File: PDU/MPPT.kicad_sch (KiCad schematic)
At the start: 13 parts, among them J3 Screw_Terminal_01x02, J4 Conn_01x03_Socket, J5 Conn_01x02_Socket, U8 MAX20801TPBA+

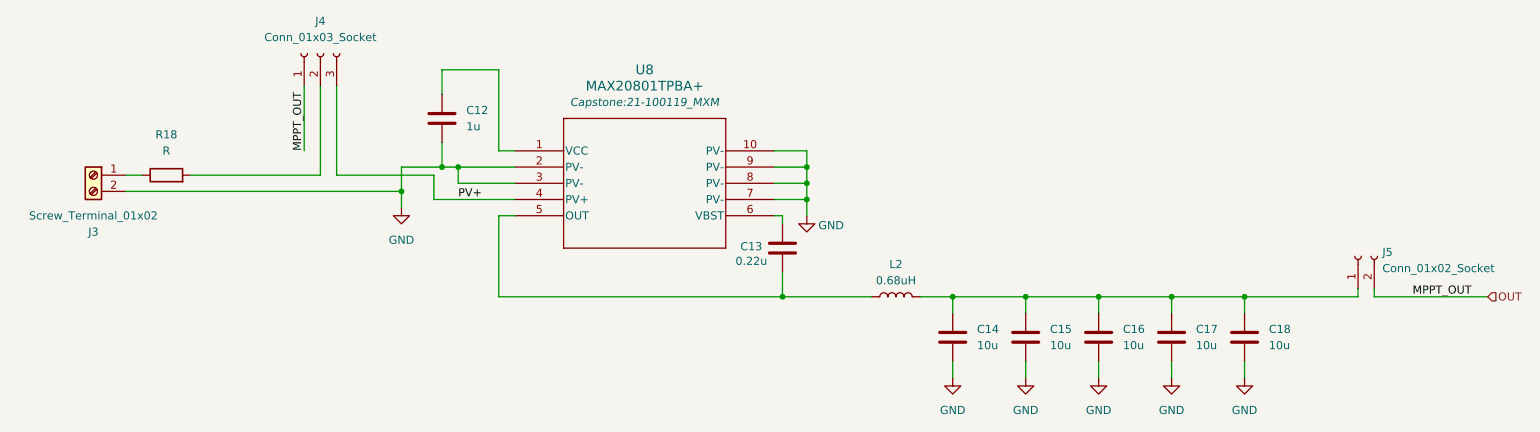
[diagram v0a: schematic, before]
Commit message: Last revision
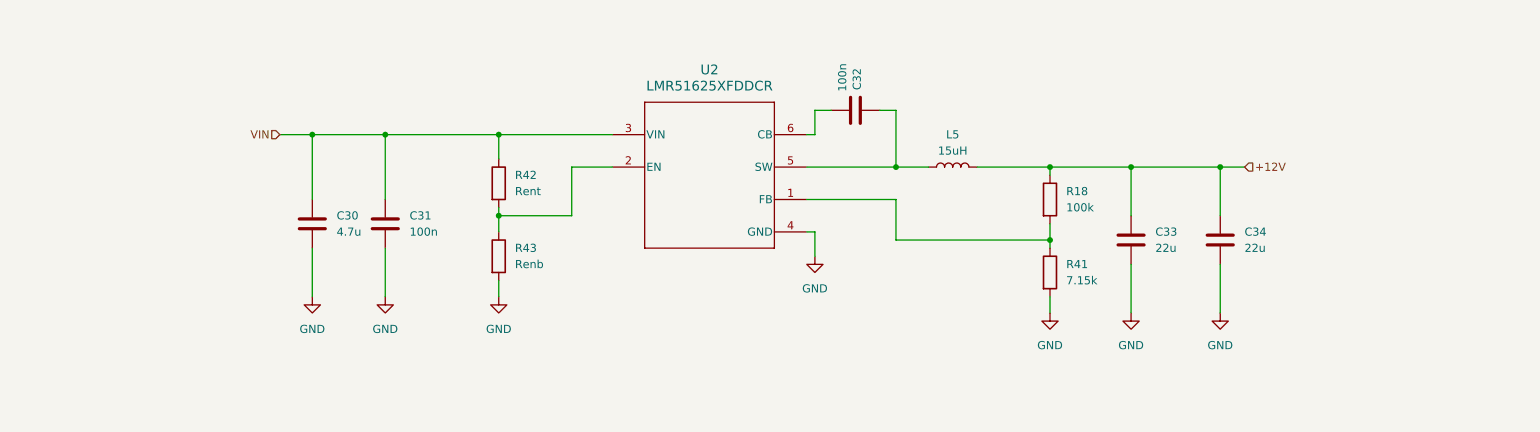
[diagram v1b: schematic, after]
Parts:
- removed C12: 1u, Capacitor_SMD:C_1206_3216Metric_Pad1.33x1.80mm_HandSolder, symbol Device:C
- removed C13: 0.22u, Capacitor_SMD:C_1206_3216Metric_Pad1.33x1.80mm_HandSolder, symbol Device:C
- removed C14, C15, C16, C17, C18: 10u, Capacitor_SMD:C_1206_3216Metric_Pad1.33x1.80mm_HandSolder, symbol Device:C
- removed J3: Screw_Terminal_01x02, TerminalBlock:TerminalBlock_Altech_AK300-2_P5.00mm, symbol Connector:Screw_Terminal_01x02
- removed J4: Conn_01x03_Socket, Connector_PinHeader_2.54mm:PinHeader_1x03_P2.54mm_Vertical, symbol Connector:Conn_01x03_Socket
- removed J5: Conn_01x02_Socket, Connector_PinHeader_2.54mm:PinHeader_1x02_P2.54mm_Vertical, symbol Connector:Conn_01x02_Socket
- removed L2: 0.68uH, Capstone:IND_RR68M8A_VIS, symbol Device:L
- removed U8: MAX20801TPBA+, Capstone:21-100119_MXM, symbol Capstone:MAX20801TPBA+
- added C30: 4.7u, Capacitor_SMD:C_1206_3216Metric_Pad1.33x1.80mm_HandSolder, symbol Device:C
- added C31, C32: 100n, Capacitor_SMD:C_1206_3216Metric_Pad1.33x1.80mm_HandSolder, symbol Device:C
- added C33, C34: 22u, Capacitor_SMD:C_1206_3216Metric_Pad1.33x1.80mm_HandSolder, symbol Device:C
- added L5: 15uH, Capstone:IND_BOURNS_SRR1208, symbol Device:L
- added R41: 7.15k, Resistor_SMD:R_1206_3216Metric_Pad1.30x1.75mm_HandSolder, symbol Device:R
- added R42: Rent, Resistor_SMD:R_1206_3216Metric_Pad1.30x1.75mm_HandSolder, symbol Device:R
- added R43: Renb, Resistor_SMD:R_1206_3216Metric_Pad1.30x1.75mm_HandSolder, symbol Device:R
- added U2: LMR51625XFDDCR, Capstone:DDC0006A-MFG, symbol Capstone:LMR51625XFDDCR
- R18: value R -> 100k; footprint Resistor_THT:R_Axial_DIN0309_L9.0mm_D3.2mm_P15.24mm_Horizontal -> Resistor_SMD:R_1206_3216Metric_Pad1.30x1.75mm_HandSolder
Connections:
- net GND: now also C30.2, C31.2, C33.2, C34.2, R41.2, R43.2, U2.4 (GND)
- net +12V: now reaches R18.1
- net +12V: now also C33.1, C34.1, L5.2
- net at R18.2: now also R41.1, U2.1 (FB)
- new net: C32.1, L5.1, U2.5 (SW)
- new net: C32.2, U2.6 (CB)
- new net: R42.2, R43.1, U2.2 (EN)
- new net VIN: C30.1, C31.1, R42.1, U2.3 (VIN)
